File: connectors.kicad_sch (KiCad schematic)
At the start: 4 parts

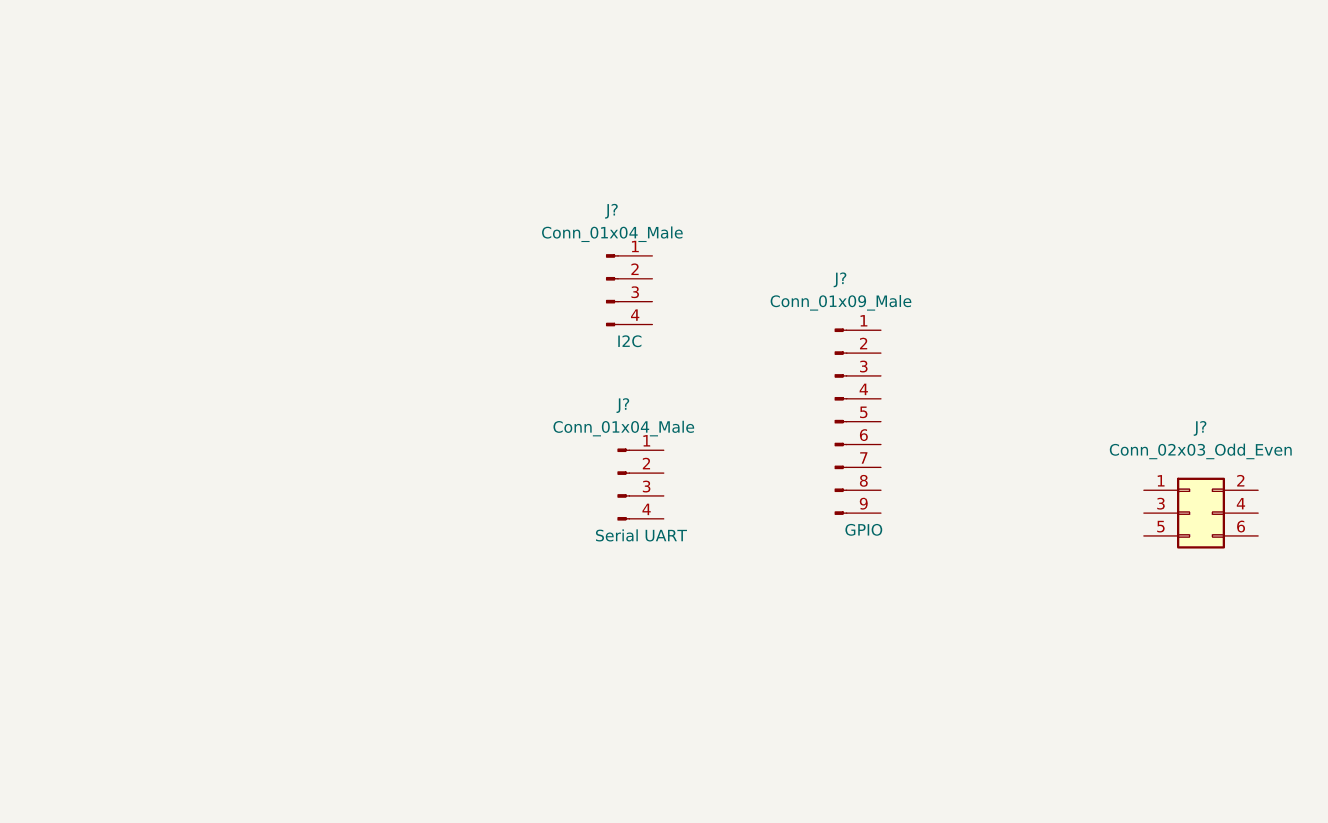
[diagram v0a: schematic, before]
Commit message: Schematic design complete
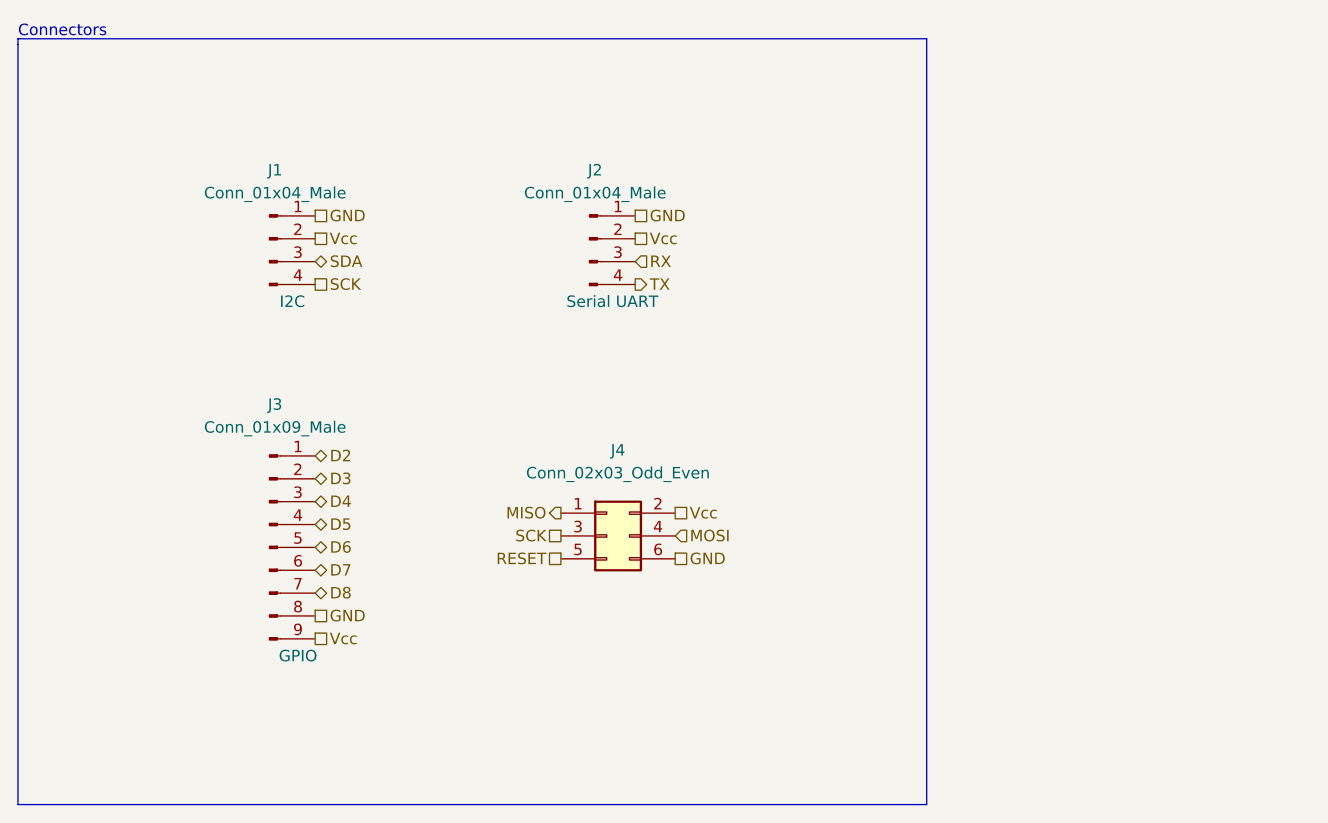
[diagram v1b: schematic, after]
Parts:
- J1, J2: renamed from J?; footprint (none) -> Connector_PinHeader_2.54mm:PinHeader_1x04_P2.54mm_Vertical
- J3: renamed from J?; footprint (none) -> Connector_PinHeader_2.54mm:PinHeader_1x09_P2.54mm_Vertical
- J4: renamed from J?; footprint (none) -> Connector_PinHeader_2.54mm:PinHeader_2x03_P2.54mm_Vertical
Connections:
- net MISO: now reaches J4.1 (Pin_1)
- net Vcc: now reaches J4.2 (Pin_2)
- net Vcc: now also J1.2 (Pin_2), J2.2 (Pin_2), J3.9 (Pin_9)
- net SCK: now reaches J4.3 (Pin_3)
- net SCK: now also J1.4 (Pin_4)
- net MOSI: now reaches J4.4 (Pin_4)
- net RESET: now reaches J4.5 (Pin_5)
- net GND: now reaches J4.6 (Pin_6)
- net GND: now also J1.1 (Pin_1), J2.1 (Pin_1), J3.8 (Pin_8)
- net D2: now reaches J3.1 (Pin_1)
- net D3: now reaches J3.2 (Pin_2)
- net D4: now reaches J3.3 (Pin_3)
- net D5: now reaches J3.4 (Pin_4)
- net D6: now reaches J3.5 (Pin_5)
- net D7: now reaches J3.6 (Pin_6)
- net D8: now reaches J3.7 (Pin_7)
- net SDA: now reaches J1.3 (Pin_3)
- net RX: now reaches J2.3 (Pin_3)
- net TX: now reaches J2.4 (Pin_4)
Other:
- note added: "Connectors"
- title: (none) -> ${project_name}
- moved on the sheet: J1, J2, J3, J4
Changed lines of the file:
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@@
 (kicad_sch (version 20211123) (generator eeschema)
   (paper "A4")
-  (symbol (lib_id "Connector_Generic:Conn_02x03_Odd_Even") (at 222.25 112.395 0) (unit 1)
+  (title_block
+    (title "${project_name}")
+    (date "2022-08-29")
+    (rev "1")
+    (comment 1 "Project #2, KiCad Like a Pro Udemy course")
+    (comment 2 "MCU Datalogger with memory and clock")
+    (comment 3 "github.com/raghavmarwah")
+    (comment 4 "raghavmarwah.com")
+  )
+  (polyline (pts (xy 193.04 59.69) (xy 193.04 144.78))
+    (stroke (width 0) (type default) (color 0 0 0 0))
+  )
+  (polyline (pts (xy 92.075 59.69) (xy 92.075 60.325))
+    (stroke (width 0) (type default) (color 0 0 0 0))
+  )
+  (polyline (pts (xy 92.075 60.325) (xy 92.075 144.78))
+    (stroke (width 0) (type default) (color 0 0 0 0))
+  )
+  (polyline (pts (xy 92.075 144.78) (xy 193.04 144.78))
+    (stroke (width 0) (type default) (color 0 0 0 0))
+  )
+  (polyline (pts (xy 193.04 59.69) (xy 92.075 59.69))
+    (stroke (width 0) (type default) (color 0 0 0 0))
+  )
+  (text "Connectors" (at 92.075 59.69 0)
+    (effects (font (size 1.27 1.27)) (justify left bottom))
+  )
+  (hierarchical_label "Vcc" (shape passive) (at 125.095 81.915 0)
+    (effects (font (size 1.27 1.27)) (justify left))
+  )
+  (hierarchical_label "GND" (shape passive) (at 160.655 79.375 0)
+    (effects (font (size 1.27 1.27)) (justify left))
+  )
+  (hierarchical_label "D4" (shape bidirectional) (at 125.095 111.125 0)
+    (effects (font (size 1.27 1.27)) (justify left))
+  )
+  (hierarchical_label "Vcc" (shape passive) (at 160.655 81.915 0)
+    (effects (font (size 1.27 1.27)) (justify left))
+  )
+  (hierarchical_label "SCK" (shape passive) (at 125.095 86.995 0)
+    (effects (font (size 1.27 1.27)) (justify left))
+  )
+  (hierarchical_label "SCK" (shape passive) (at 152.4 114.935 180)
+    (effects (font (size 1.27 1.27)) (justify right))
+  )
+  (hierarchical_label "D6" (shape bidirectional) (at 125.095 116.205 0)
+    (effects (font (size 1.27 1.27)) (justify left))
+  )
+  (hierarchical_label "GND" (shape passive) (at 165.1 117.475 0)
+    (effects (font (size 1.27 1.27)) (justify left))
+  )
+  (hierarchical_label "GND" (shape passive) (at 125.095 123.825 0)
+    (effects (font (size 1.27 1.27)) (justify left))
+  )
+  (hierarchical_label "D2" (shape bidirectional) (at 125.095 106.045 0)
+    (effects (font (size 1.27 1.27)) (justify left))
+  )
+  (hierarchical_label "TX" (shape output) (at 160.655 86.995 0)
+    (effects (font (size 1.27 1.27)) (justify left))
+  )
+  (hierarchical_label "SDA" (shape bidirectional) (at 125.095 84.455 0)
+    (effects (font (size 1.27 1.27)) (justify left))
+  )
+  (hierarchical_label "D3" (shape bidirectional) (at 125.095 108.585 0)
+    (effects (font (size 1.27 1.27)) (justify left))
+  )
+  (hierarchical_label "RESET" (shape passive) (at 152.4 117.475 180)
+    (effects (font (size 1.27 1.27)) (justify right))
+  )
+  (hierarchical_label "Vcc" (shape passive) (at 125.095 126.365 0)
+    (effects (font (size 1.27 1.27)) (justify left))
+  )
+  (hierarchical_label "D5" (shape bidirectional) (at 125.095 113.665 0)
+    (effects (font (size 1.27 1.27)) (justify left))
+  )
+  (hierarchical_label "D8" (shape bidirectional) (at 125.095 121.285 0)
+    (effects (font (size 1.27 1.27)) (justify left))
+  )
+  (hierarchical_label "MOSI" (shape input) (at 165.1 114.935 0)
+    (effects (font (size 1.27 1.27)) (justify left))
+  )
+  (hierarchical_label "D7" (shape bidirectional) (at 125.095 118.745 0)
+    (effects (font (size 1.27 1.27)) (justify left))
+  )
+  (hierarchical_label "RX" (shape input) (at 160.655 84.455 0)
+    (effects (font (size 1.27 1.27)) (justify left))
+  )
+  (hierarchical_label "Vcc" (shape passive) (at 165.1 112.395 0)
+    (effects (font (size 1.27 1.27)) (justify left))
+  )
+  (hierarchical_label "MISO" (shape output) (at 152.4 112.395 180)
+    (effects (font (size 1.27 1.27)) (justify right))
+  )
+  (hierarchical_label "GND" (shape passive) (at 125.095 79.375 0)
+    (effects (font (size 1.27 1.27)) (justify left))
+  )
+  (symbol (lib_id "Connector_Generic:Conn_02x03_Odd_Even") (at 157.48 114.935 0) (unit 1)
     (in_bom yes) (on_board yes) (fields_autoplaced)
-    (property "Reference" "J?" (id 0) (at 223.52 102.87 0))
-    (property "Value" "Conn_02x03_Odd_Even" (id 1) (at 223.52 105.41 0))
-    (property "Footprint" "" (id 2) (at 222.25 112.395 0)
+    (property "Reference" "J4" (id 0) (at 158.75 105.41 0))
+    (property "Value" "Conn_02x03_Odd_Even" (id 1) (at 158.75 107.95 0))
+    (property "Footprint" "Connector_PinHeader_2.54mm:PinHeader_2x03_P2.54mm_Vertical" (id 2) (at 157.48 114.935 0)
       (effects (font (size 1.27 1.27)) hide)
     )
-    (property "Datasheet" "~" (id 3) (at 222.25 112.395 0)
+    (property "Datasheet" "~" (id 3) (at 157.48 114.935 0)
       (effects (font (size 1.27 1.27)) hide)
     )
@@
     (pin "6")
   )
-  (symbol (lib_id "Connector:Conn_01x09_Male") (at 182.88 102.235 0) (unit 1)
+  (symbol (lib_id "Connector:Conn_01x09_Male") (at 120.015 116.205 0) (unit 1)
     (in_bom yes) (on_board yes)
-    (property "Reference" "J?" (id 0) (at 183.515 86.36 0))
-    (property "Value" "Conn_01x09_Male" (id 1) (at 183.515 88.9 0))
-    (property "Footprint" "" (id 2) (at 182.88 102.235 0)
+    (property "Reference" "J3" (id 0) (at 120.65 100.33 0))
+    (property "Value" "Conn_01x09_Male" (id 1) (at 120.65 102.87 0))
+    (property "Footprint" "Connector_PinHeader_2.54mm:PinHeader_1x09_P2.54mm_Vertical" (id 2) (at 120.015 116.205 0)
       (effects (font (size 1.27 1.27)) hide)
     )
-    (property "Datasheet" "~" (id 3) (at 182.88 102.235 0)
+    (property "Datasheet" "~" (id 3) (at 120.015 116.205 0)
       (effects (font (size 1.27 1.27)) hide)
     )
-    (property "Purpose" "GPIO" (id 4) (at 186.055 114.3 0))
+    (property "Purpose" "GPIO" (id 4) (at 123.19 128.27 0))
     (pin "1")
     (pin "2")
@@
     (pin "9")
   )
-  (symbol (lib_id "Connector:Conn_01x04_Male") (at 157.48 86.36 0) (unit 1)
+  (symbol (lib_id "Connector:Conn_01x04_Male") (at 120.015 81.915 0) (unit 1)
     (in_bom yes) (on_board yes)
-    (property "Reference" "J?" (id 0) (at 158.115 78.74 0))
-    (property "Value" "Conn_01x04_Male" (id 1) (at 158.115 81.28 0))
-    (property "Footprint" "" (id 2) (at 157.48 86.36 0)
+    (property "Reference" "J1" (id 0) (at 120.65 74.295 0))
+    (property "Value" "Conn_01x04_Male" (id 1) (at 120.65 76.835 0))
+    (property "Footprint" "Connector_PinHeader_2.54mm:PinHeader_1x04_P2.54mm_Vertical" (id 2) (at 120.015 81.915 0)
       (effects (font (size 1.27 1.27)) hide)
     )
-    (property "Datasheet" "~" (id 3) (at 157.48 86.36 0)
+    (property "Datasheet" "~" (id 3) (at 120.015 81.915 0)
       (effects (font (size 1.27 1.27)) hide)
     )
-    (property "Purpose" "I2C" (id 4) (at 160.02 93.345 0))
+    (property "Purpose" "I2C" (id 4) (at 122.555 88.9 0))
     (pin "1")
     (pin "2")
@@
     (pin "4")
   )
-  (symbol (lib_id "Connector:Conn_01x04_Male") (at 158.75 107.95 0) (unit 1)
+  (symbol (lib_id "Connector:Conn_01x04_Male") (at 155.575 81.915 0) (unit 1)
     (in_bom yes) (on_board yes)
-    (property "Reference" "J?" (id 0) (at 159.385 100.33 0))
-    (property "Value" "Conn_01x04_Male" (id 1) (at 159.385 102.87 0))
-    (property "Footprint" "" (id 2) (at 158.75 107.95 0)
+    (property "Reference" "J2" (id 0) (at 156.21 74.295 0))
+    (property "Value" "Conn_01x04_Male" (id 1) (at 156.21 76.835 0))
+    (property "Footprint" "Connector_PinHeader_2.54mm:PinHeader_1x04_P2.54mm_Vertical" (id 2) (at 155.575 81.915 0)
       (effects (font (size 1.27 1.27)) hide)
     )
-    (property "Datasheet" "~" (id 3) (at 158.75 107.95 0)
+    (property "Datasheet" "~" (id 3) (at 155.575 81.915 0)
       (effects (font (size 1.27 1.27)) hide)
     )
-    (property "Purpose" "Serial UART" (id 4) (at 161.29 114.935 0))
+    (property "Purpose" "Serial UART" (id 4) (at 158.115 88.9 0))
     (pin "1")
     (pin "2")
